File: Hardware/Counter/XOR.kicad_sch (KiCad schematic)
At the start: 12 parts, among them Q117 FDN335N, Q118 FDN360P, Q119 FDN335N, Q120 FDN335N, Q121 FDN360P, Q122 FDN335N, Q123 FDN335N, Q124 FDN335N, U66 FDN360P, U67 FDN360P, U68 FDN360P, U69 FDN360P

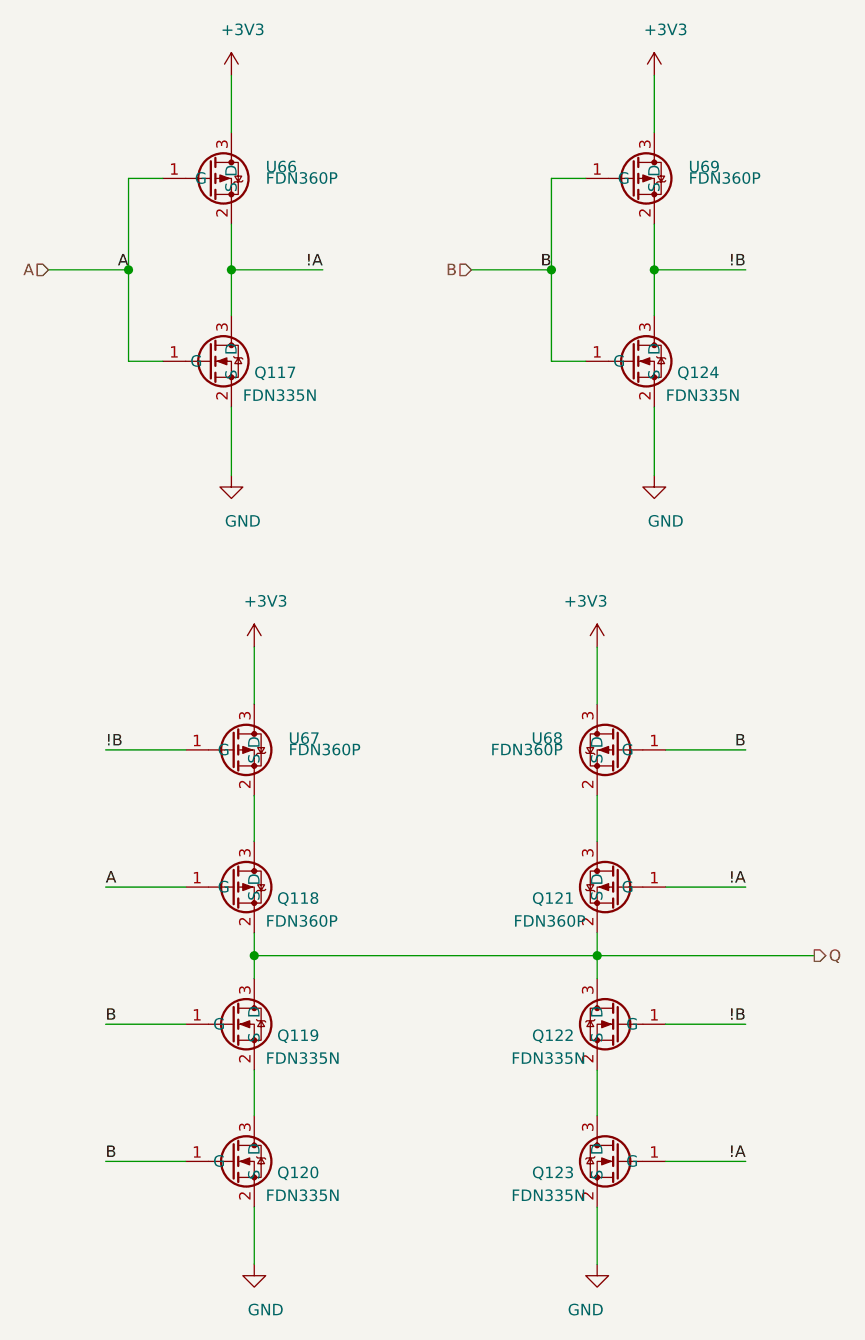
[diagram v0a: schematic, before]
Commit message: working on connectin bits together
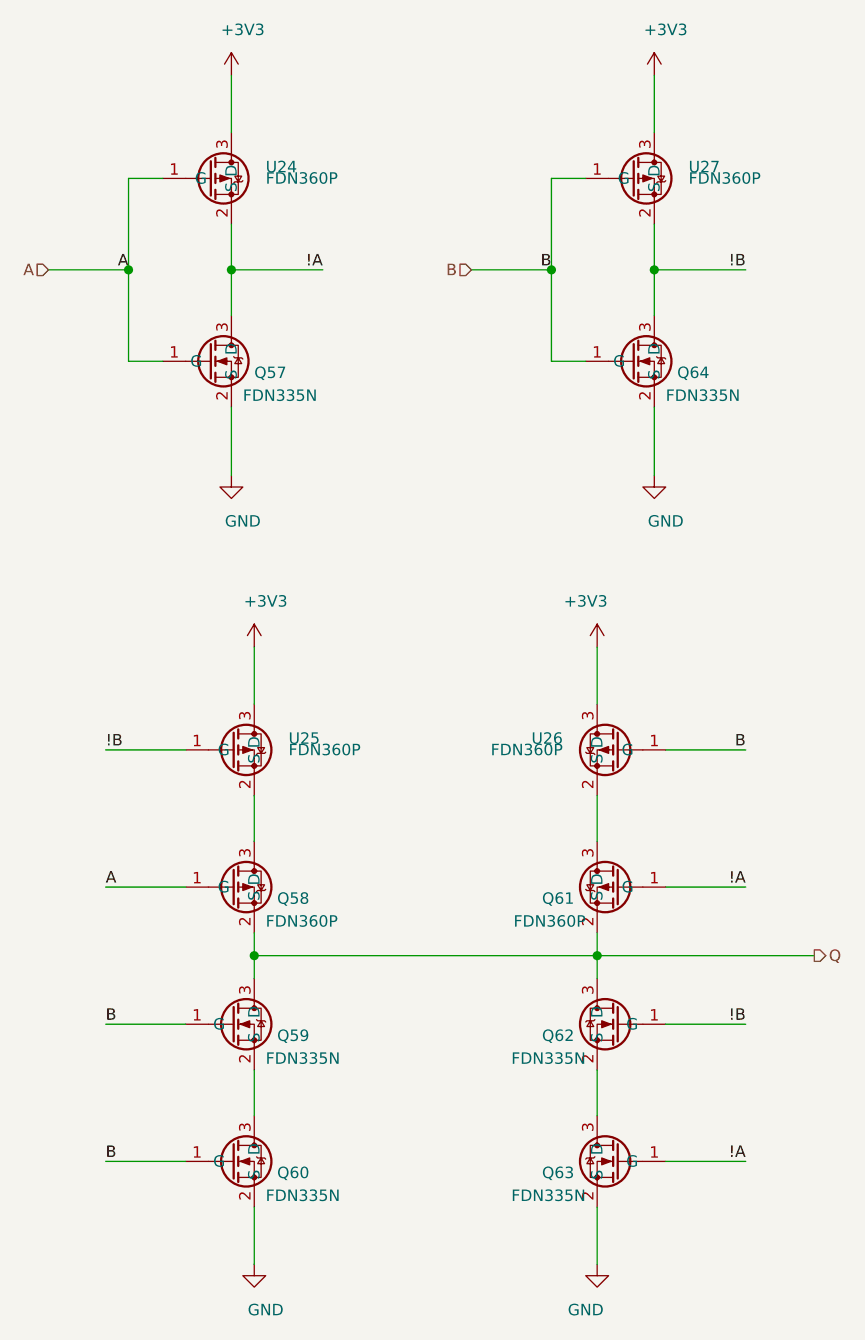
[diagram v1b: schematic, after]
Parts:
- renumbered Q117 to Q57, Q118 to Q58, Q119 to Q59, Q120 to Q60, Q121 to Q61, Q122 to Q62, Q123 to Q63, Q124 to Q64, U66 to U24, U67 to U25, U68 to U26, U69 to U27
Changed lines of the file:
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@@
   (symbol (lib_id "power:+3V3") (at 121.92 19.05 0)
     (in_bom yes) (on_board yes)
-    (property "Reference" "#PWR0247" (id 0) (at 121.92 22.86 0)
+    (property "Reference" "#PWR0176" (id 0) (at 121.92 22.86 0)
       (effects (font (size 1.27 1.27)) hide)
     )
@@
   (symbol (lib_id "power:+3V3") (at 124.46 82.55 0)
     (in_bom yes) (on_board yes)
-    (property "Reference" "#PWR0248" (id 0) (at 124.46 86.36 0)
+    (property "Reference" "#PWR0177" (id 0) (at 124.46 86.36 0)
       (effects (font (size 1.27 1.27)) hide)
     )
@@
   (symbol (lib_id "power:+3V3") (at 162.56 82.55 0) (mirror y)
     (in_bom yes) (on_board yes)
-    (property "Reference" "#PWR0251" (id 0) (at 162.56 86.36 0)
+    (property "Reference" "#PWR0180" (id 0) (at 162.56 86.36 0)
       (effects (font (size 1.27 1.27)) hide)
     )
@@
   (symbol (lib_id "power:+3V3") (at 168.91 19.05 0)
     (in_bom yes) (on_board yes)
-    (property "Reference" "#PWR0246" (id 0) (at 168.91 22.86 0)
+    (property "Reference" "#PWR0175" (id 0) (at 168.91 22.86 0)
       (effects (font (size 1.27 1.27)) hide)
     )
@@
   (symbol (lib_id "power:GND") (at 121.92 63.5 0)
     (in_bom yes) (on_board yes)
-    (property "Reference" "#PWR0245" (id 0) (at 121.92 69.85 0)
+    (property "Reference" "#PWR0174" (id 0) (at 121.92 69.85 0)
       (effects (font (size 1.27 1.27)) hide)
     )
@@
   (symbol (lib_id "power:GND") (at 124.46 151.13 0)
     (in_bom yes) (on_board yes)
-    (property "Reference" "#PWR0250" (id 0) (at 124.46 157.48 0)
+    (property "Reference" "#PWR0179" (id 0) (at 124.46 157.48 0)
       (effects (font (size 1.27 1.27)) hide)
     )
@@
   (symbol (lib_id "power:GND") (at 162.56 151.13 0) (mirror y)
     (in_bom yes) (on_board yes)
-    (property "Reference" "#PWR0249" (id 0) (at 162.56 157.48 0)
+    (property "Reference" "#PWR0178" (id 0) (at 162.56 157.48 0)
       (effects (font (size 1.27 1.27)) hide)
     )
@@
   (symbol (lib_id "power:GND") (at 168.91 63.5 0)
     (in_bom yes) (on_board yes)
-    (property "Reference" "#PWR0244" (id 0) (at 168.91 69.85 0)
+    (property "Reference" "#PWR0173" (id 0) (at 168.91 69.85 0)
       (effects (font (size 1.27 1.27)) hide)
     )
@@
   (symbol (lib_name "Custom_Transistors:FDN360P_1") (lib_id "Custom_Transistors:FDN360P") (at 121.92 30.48 0)
     (in_bom yes) (on_board yes)
-    (property "Reference" "U66" (id 0) (at 125.73 29.21 0)
+    (property "Reference" "U24" (id 0) (at 125.73 29.21 0)
       (effects (font (size 1.27 1.27)) (justify left))
     )
@@
   (symbol (lib_id "Custom_Transistors:FDN335N") (at 121.92 50.8 0)
     (in_bom yes) (on_board yes)
-    (property "Reference" "Q117" (id 0) (at 124.46 52.07 0)
+    (property "Reference" "Q57" (id 0) (at 124.46 52.07 0)
       (effects (font (size 1.27 1.27)) (justify left))
     )
@@
   (symbol (lib_name "Custom_Transistors:FDN360P_2") (lib_id "Custom_Transistors:FDN360P") (at 124.46 93.98 0)
     (in_bom yes) (on_board yes)
-    (property "Reference" "U67" (id 0) (at 128.27 92.71 0)
+    (property "Reference" "U25" (id 0) (at 128.27 92.71 0)
       (effects (font (size 1.27 1.27)) (justify left))
     )
@@
   (symbol (lib_name "Custom_Transistors:FDN360P_3") (lib_id "Custom_Transistors:FDN360P") (at 124.46 109.22 0)
     (in_bom yes) (on_board yes)
-    (property "Reference" "Q118" (id 0) (at 127 110.49 0)
+    (property "Reference" "Q58" (id 0) (at 127 110.49 0)
       (effects (font (size 1.27 1.27)) (justify left))
     )
@@
   (symbol (lib_id "Custom_Transistors:FDN335N") (at 124.46 124.46 0)
     (in_bom yes) (on_board yes)
-    (property "Reference" "Q119" (id 0) (at 127 125.73 0)
+    (property "Reference" "Q59" (id 0) (at 127 125.73 0)
       (effects (font (size 1.27 1.27)) (justify left))
     )
@@
   (symbol (lib_id "Custom_Transistors:FDN335N") (at 124.46 139.7 0)
     (in_bom yes) (on_board yes)
-    (property "Reference" "Q120" (id 0) (at 127 140.97 0)
+    (property "Reference" "Q60" (id 0) (at 127 140.97 0)
       (effects (font (size 1.27 1.27)) (justify left))
     )
@@
   (symbol (lib_name "Custom_Transistors:FDN360P_4") (lib_id "Custom_Transistors:FDN360P") (at 162.56 93.98 0) (mirror y)
     (in_bom yes) (on_board yes)
-    (property "Reference" "U68" (id 0) (at 158.75 92.71 0)
+    (property "Reference" "U26" (id 0) (at 158.75 92.71 0)
       (effects (font (size 1.27 1.27)) (justify left))
     )
@@
   (symbol (lib_name "Custom_Transistors:FDN360P_5") (lib_id "Custom_Transistors:FDN360P") (at 162.56 109.22 0) (mirror y)
     (in_bom yes) (on_board yes)
-    (property "Reference" "Q121" (id 0) (at 160.02 110.49 0)
+    (property "Reference" "Q61" (id 0) (at 160.02 110.49 0)
       (effects (font (size 1.27 1.27)) (justify left))
     )
@@
   (symbol (lib_id "Custom_Transistors:FDN335N") (at 162.56 124.46 0) (mirror y)
     (in_bom yes) (on_board yes)
-    (property "Reference" "Q122" (id 0) (at 160.02 125.73 0)
+    (property "Reference" "Q62" (id 0) (at 160.02 125.73 0)
       (effects (font (size 1.27 1.27)) (justify left))
     )
@@
   (symbol (lib_id "Custom_Transistors:FDN335N") (at 162.56 139.7 0) (mirror y)
     (in_bom yes) (on_board yes)
-    (property "Reference" "Q123" (id 0) (at 160.02 140.97 0)
+    (property "Reference" "Q63" (id 0) (at 160.02 140.97 0)
       (effects (font (size 1.27 1.27)) (justify left))
     )
@@
   (symbol (lib_id "Custom_Transistors:FDN360P") (at 168.91 30.48 0)
     (in_bom yes) (on_board yes)
-    (property "Reference" "U69" (id 0) (at 172.72 29.21 0)
+    (property "Reference" "U27" (id 0) (at 172.72 29.21 0)
       (effects (font (size 1.27 1.27)) (justify left))
     )
@@
   (symbol (lib_id "Custom_Transistors:FDN335N") (at 168.91 50.8 0)
     (in_bom yes) (on_board yes)
-    (property "Reference" "Q124" (id 0) (at 171.45 52.07 0)
-      (effects (font (size 1.27 1.27)) (justify left))
-    )
+    (property "Reference" "Q64" (id 0) (at 171.45 52.07 0)
+      (effects (font (size 1.27 1.27)) (justify left))
+    )

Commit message: kicad updates
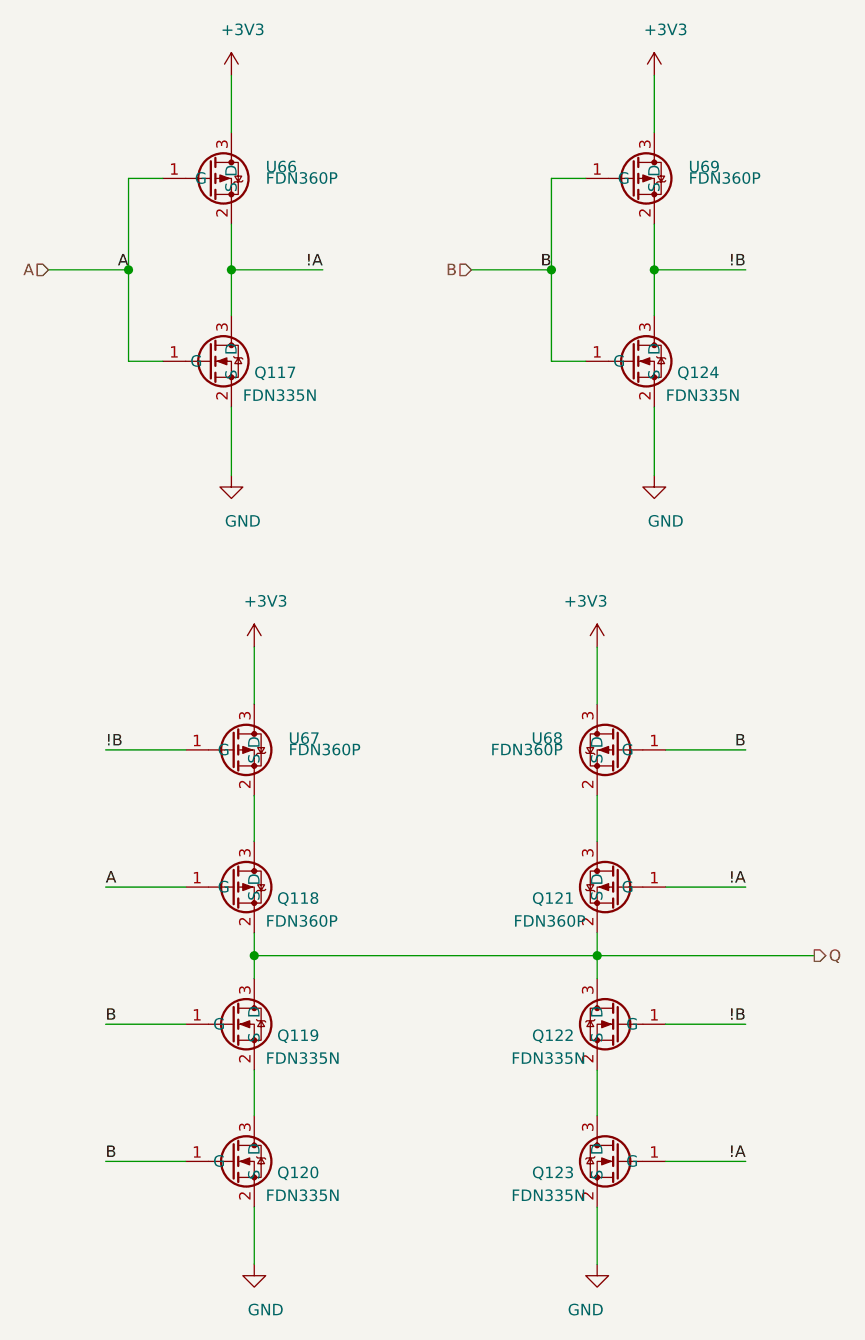
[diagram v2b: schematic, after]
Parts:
- renumbered Q57 to Q117, Q58 to Q118, Q59 to Q119, Q60 to Q120, Q61 to Q121, Q62 to Q122, Q63 to Q123, Q64 to Q124, U24 to U66, U25 to U67, U26 to U68, U27 to U69
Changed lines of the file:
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@@
   (symbol (lib_id "power:+3V3") (at 121.92 19.05 0)
     (in_bom yes) (on_board yes)
-    (property "Reference" "#PWR0176" (id 0) (at 121.92 22.86 0)
+    (property "Reference" "#PWR0247" (id 0) (at 121.92 22.86 0)
       (effects (font (size 1.27 1.27)) hide)
     )
@@
   (symbol (lib_id "power:+3V3") (at 124.46 82.55 0)
     (in_bom yes) (on_board yes)
-    (property "Reference" "#PWR0177" (id 0) (at 124.46 86.36 0)
+    (property "Reference" "#PWR0248" (id 0) (at 124.46 86.36 0)
       (effects (font (size 1.27 1.27)) hide)
     )
@@
   (symbol (lib_id "power:+3V3") (at 162.56 82.55 0) (mirror y)
     (in_bom yes) (on_board yes)
-    (property "Reference" "#PWR0180" (id 0) (at 162.56 86.36 0)
+    (property "Reference" "#PWR0251" (id 0) (at 162.56 86.36 0)
       (effects (font (size 1.27 1.27)) hide)
     )
@@
   (symbol (lib_id "power:+3V3") (at 168.91 19.05 0)
     (in_bom yes) (on_board yes)
-    (property "Reference" "#PWR0175" (id 0) (at 168.91 22.86 0)
+    (property "Reference" "#PWR0246" (id 0) (at 168.91 22.86 0)
       (effects (font (size 1.27 1.27)) hide)
     )
@@
   (symbol (lib_id "power:GND") (at 121.92 63.5 0)
     (in_bom yes) (on_board yes)
-    (property "Reference" "#PWR0174" (id 0) (at 121.92 69.85 0)
+    (property "Reference" "#PWR0245" (id 0) (at 121.92 69.85 0)
       (effects (font (size 1.27 1.27)) hide)
     )
@@
   (symbol (lib_id "power:GND") (at 124.46 151.13 0)
     (in_bom yes) (on_board yes)
-    (property "Reference" "#PWR0179" (id 0) (at 124.46 157.48 0)
+    (property "Reference" "#PWR0250" (id 0) (at 124.46 157.48 0)
       (effects (font (size 1.27 1.27)) hide)
     )
@@
   (symbol (lib_id "power:GND") (at 162.56 151.13 0) (mirror y)
     (in_bom yes) (on_board yes)
-    (property "Reference" "#PWR0178" (id 0) (at 162.56 157.48 0)
+    (property "Reference" "#PWR0249" (id 0) (at 162.56 157.48 0)
       (effects (font (size 1.27 1.27)) hide)
     )
@@
   (symbol (lib_id "power:GND") (at 168.91 63.5 0)
     (in_bom yes) (on_board yes)
-    (property "Reference" "#PWR0173" (id 0) (at 168.91 69.85 0)
+    (property "Reference" "#PWR0244" (id 0) (at 168.91 69.85 0)
       (effects (font (size 1.27 1.27)) hide)
     )
@@
   (symbol (lib_name "Custom_Transistors:FDN360P_1") (lib_id "Custom_Transistors:FDN360P") (at 121.92 30.48 0)
     (in_bom yes) (on_board yes)
-    (property "Reference" "U24" (id 0) (at 125.73 29.21 0)
+    (property "Reference" "U66" (id 0) (at 125.73 29.21 0)
       (effects (font (size 1.27 1.27)) (justify left))
     )
@@
   (symbol (lib_id "Custom_Transistors:FDN335N") (at 121.92 50.8 0)
     (in_bom yes) (on_board yes)
-    (property "Reference" "Q57" (id 0) (at 124.46 52.07 0)
+    (property "Reference" "Q117" (id 0) (at 124.46 52.07 0)
       (effects (font (size 1.27 1.27)) (justify left))
     )
@@
   (symbol (lib_name "Custom_Transistors:FDN360P_2") (lib_id "Custom_Transistors:FDN360P") (at 124.46 93.98 0)
     (in_bom yes) (on_board yes)
-    (property "Reference" "U25" (id 0) (at 128.27 92.71 0)
+    (property "Reference" "U67" (id 0) (at 128.27 92.71 0)
       (effects (font (size 1.27 1.27)) (justify left))
     )
@@
   (symbol (lib_name "Custom_Transistors:FDN360P_3") (lib_id "Custom_Transistors:FDN360P") (at 124.46 109.22 0)
     (in_bom yes) (on_board yes)
-    (property "Reference" "Q58" (id 0) (at 127 110.49 0)
+    (property "Reference" "Q118" (id 0) (at 127 110.49 0)
       (effects (font (size 1.27 1.27)) (justify left))
     )
@@
   (symbol (lib_id "Custom_Transistors:FDN335N") (at 124.46 124.46 0)
     (in_bom yes) (on_board yes)
-    (property "Reference" "Q59" (id 0) (at 127 125.73 0)
+    (property "Reference" "Q119" (id 0) (at 127 125.73 0)
       (effects (font (size 1.27 1.27)) (justify left))
     )
@@
   (symbol (lib_id "Custom_Transistors:FDN335N") (at 124.46 139.7 0)
     (in_bom yes) (on_board yes)
-    (property "Reference" "Q60" (id 0) (at 127 140.97 0)
+    (property "Reference" "Q120" (id 0) (at 127 140.97 0)
       (effects (font (size 1.27 1.27)) (justify left))
     )
@@
   (symbol (lib_name "Custom_Transistors:FDN360P_4") (lib_id "Custom_Transistors:FDN360P") (at 162.56 93.98 0) (mirror y)
     (in_bom yes) (on_board yes)
-    (property "Reference" "U26" (id 0) (at 158.75 92.71 0)
+    (property "Reference" "U68" (id 0) (at 158.75 92.71 0)
       (effects (font (size 1.27 1.27)) (justify left))
     )
@@
   (symbol (lib_name "Custom_Transistors:FDN360P_5") (lib_id "Custom_Transistors:FDN360P") (at 162.56 109.22 0) (mirror y)
     (in_bom yes) (on_board yes)
-    (property "Reference" "Q61" (id 0) (at 160.02 110.49 0)
+    (property "Reference" "Q121" (id 0) (at 160.02 110.49 0)
       (effects (font (size 1.27 1.27)) (justify left))
     )
@@
   (symbol (lib_id "Custom_Transistors:FDN335N") (at 162.56 124.46 0) (mirror y)
     (in_bom yes) (on_board yes)
-    (property "Reference" "Q62" (id 0) (at 160.02 125.73 0)
+    (property "Reference" "Q122" (id 0) (at 160.02 125.73 0)
       (effects (font (size 1.27 1.27)) (justify left))
     )
@@
   (symbol (lib_id "Custom_Transistors:FDN335N") (at 162.56 139.7 0) (mirror y)
     (in_bom yes) (on_board yes)
-    (property "Reference" "Q63" (id 0) (at 160.02 140.97 0)
+    (property "Reference" "Q123" (id 0) (at 160.02 140.97 0)
       (effects (font (size 1.27 1.27)) (justify left))
     )
@@
   (symbol (lib_id "Custom_Transistors:FDN360P") (at 168.91 30.48 0)
     (in_bom yes) (on_board yes)
-    (property "Reference" "U27" (id 0) (at 172.72 29.21 0)
+    (property "Reference" "U69" (id 0) (at 172.72 29.21 0)
       (effects (font (size 1.27 1.27)) (justify left))
     )
@@
   (symbol (lib_id "Custom_Transistors:FDN335N") (at 168.91 50.8 0)
     (in_bom yes) (on_board yes)
-    (property "Reference" "Q64" (id 0) (at 171.45 52.07 0)
-      (effects (font (size 1.27 1.27)) (justify left))
-    )
+    (property "Reference" "Q124" (id 0) (at 171.45 52.07 0)
+      (effects (font (size 1.27 1.27)) (justify left))
+    )
